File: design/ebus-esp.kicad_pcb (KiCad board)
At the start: 2 copper layers, 30.1 x 65.3 mm, 24 parts, among them J2 USB_B_Micro, J4 PROG, J5 PINS, J6 PWR, J7 UART, Q2 BC817, Q3 BC817, U5 AMS1117-3.3, U6 ESP-12F, U7 CH340G, Y1 12MHz 22pF

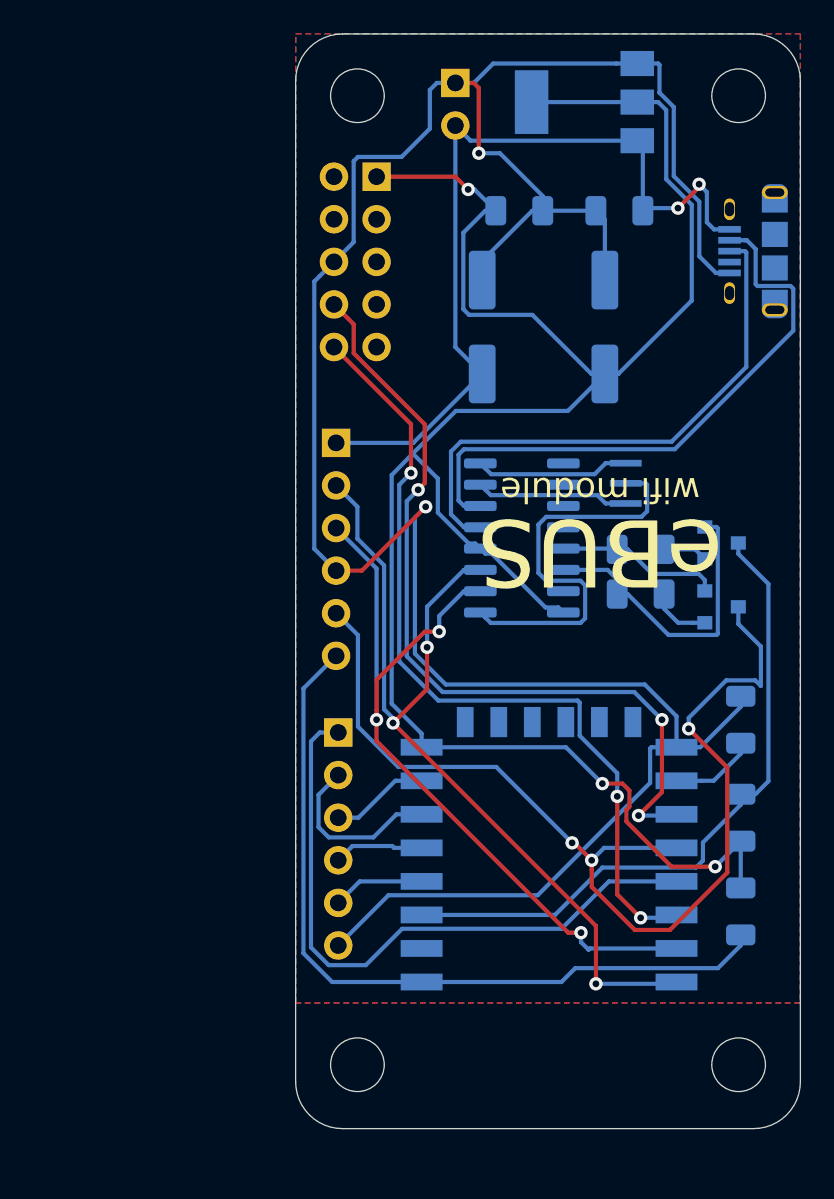
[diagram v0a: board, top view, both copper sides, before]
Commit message: usbc, updated images
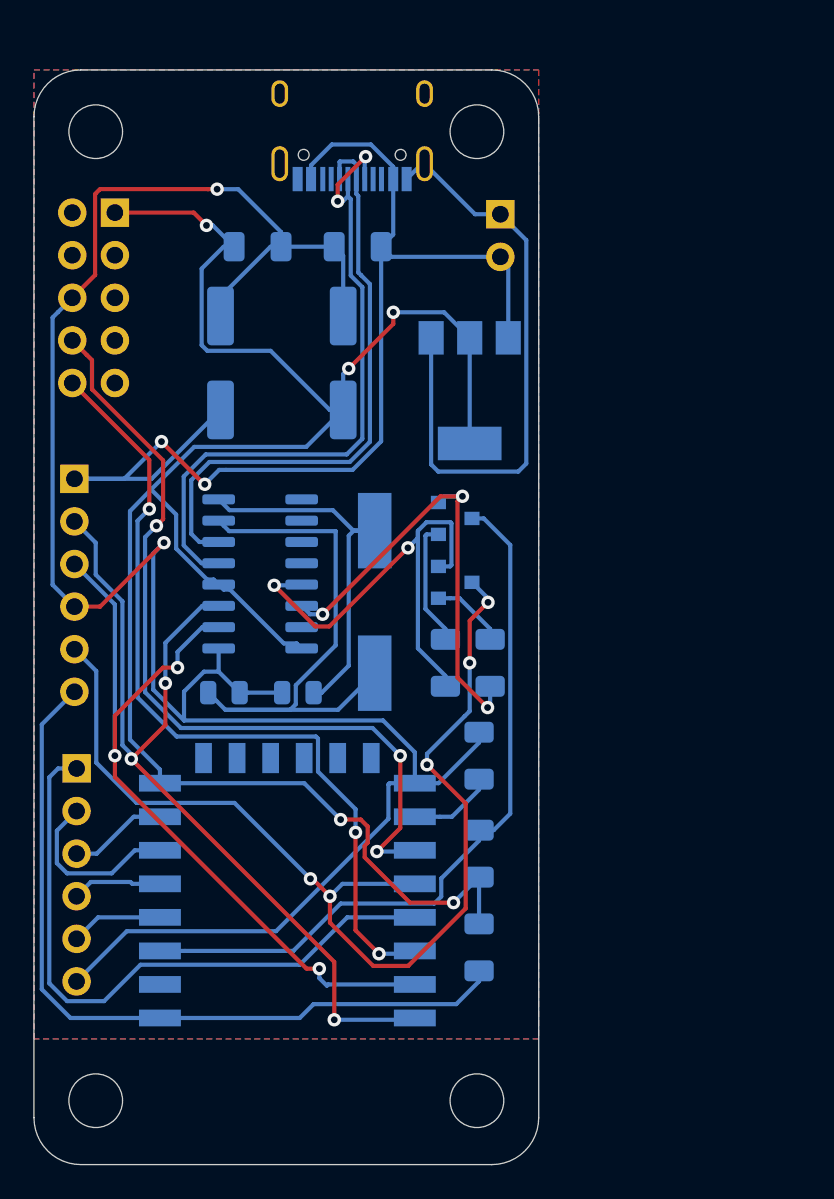
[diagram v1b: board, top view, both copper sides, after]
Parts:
- added C7: 22pF, Capacitor_SMD:C_0805_2012Metric, B.Cu at (94.3, 115.5)
- added C8: 22pF, Capacitor_SMD:C_0805_2012Metric, B.Cu at (98.7, 115.5)
- J2: value USB_B_Micro -> USB_C_Receptacle_USB2.0; footprint usb:AMPHENOL_10118194-0001LF -> Connector_USB:USB_C_Receptacle_HRO_TYPE-C-31-M-12
- Y1: value 12MHz 22pF -> Crystal; footprint Crystal:Resonator_SMD_muRata_CSTxExxV-3Pin_3.0x1.1mm -> Crystal:Crystal_SMD_HC49-SD
- moved J2 26.6 mm to (101.9, 80.8), turned to 0 degrees
- moved U5 18.5 mm to (108.9, 97.5), turned to -90 degrees
- moved Y1 16.6 mm to (103.3, 110.1)
- moved Q2 16.0 mm to (108.1, 105.1)
- moved Q3 16.0 mm to (108.1, 108.9)
- moved C3 15.8 mm to (94.1, 95.8)
- moved C4 15.8 mm to (96.3, 88.9)
- moved C5 15.8 mm to (101.4, 95.8)
- moved H5 15.8 mm to (109.4, 82.0)
- moved H6 15.8 mm to (109.4, 139.8)
- moved H7 15.8 mm to (86.6, 82.0)
- moved H8 15.8 mm to (86.6, 139.8)
- moved J4 15.8 mm to (85.4, 102.7)
- moved J5 15.8 mm to (85.5, 120.0)
- moved J7 15.8 mm to (87.8, 86.9)
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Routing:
- net (no net): track 895.4 -> 977.9 mm, vias 22 -> 33
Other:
- net class Default removed
- net class Power removed
- board text removed: "eBUS"
- board text removed: "wifi module"
- board text removed: "~"
